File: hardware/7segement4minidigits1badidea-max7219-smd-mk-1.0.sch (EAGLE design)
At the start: 12 parts, among them IC1 MAX7219

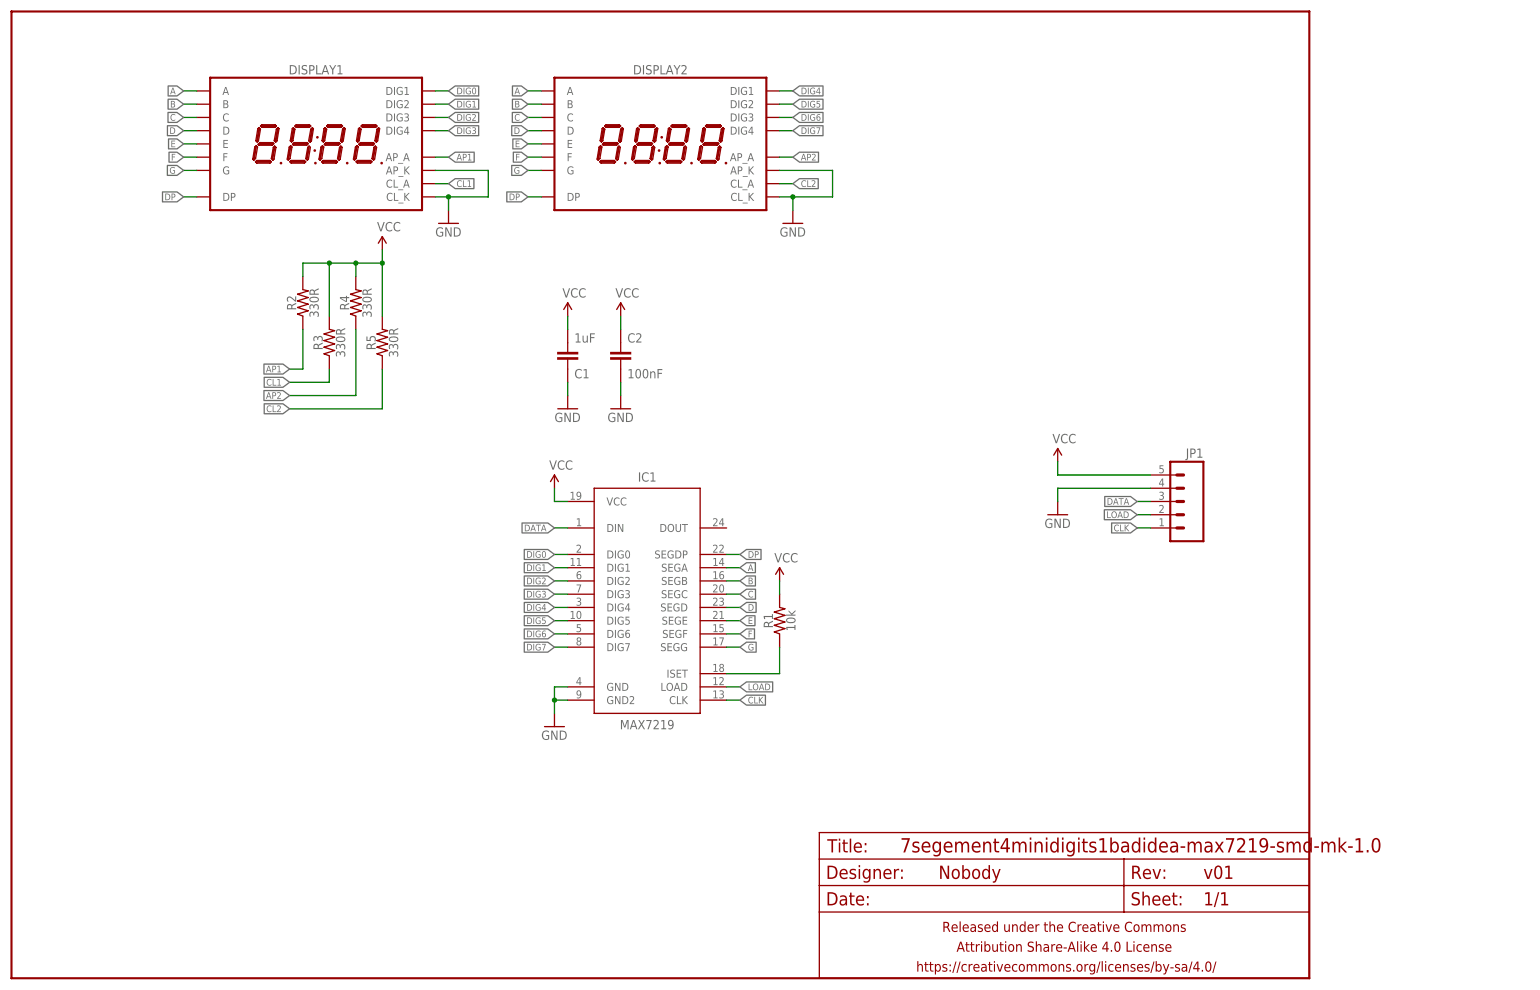
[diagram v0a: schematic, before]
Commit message: whooooole bunch of designs i apparently never committed
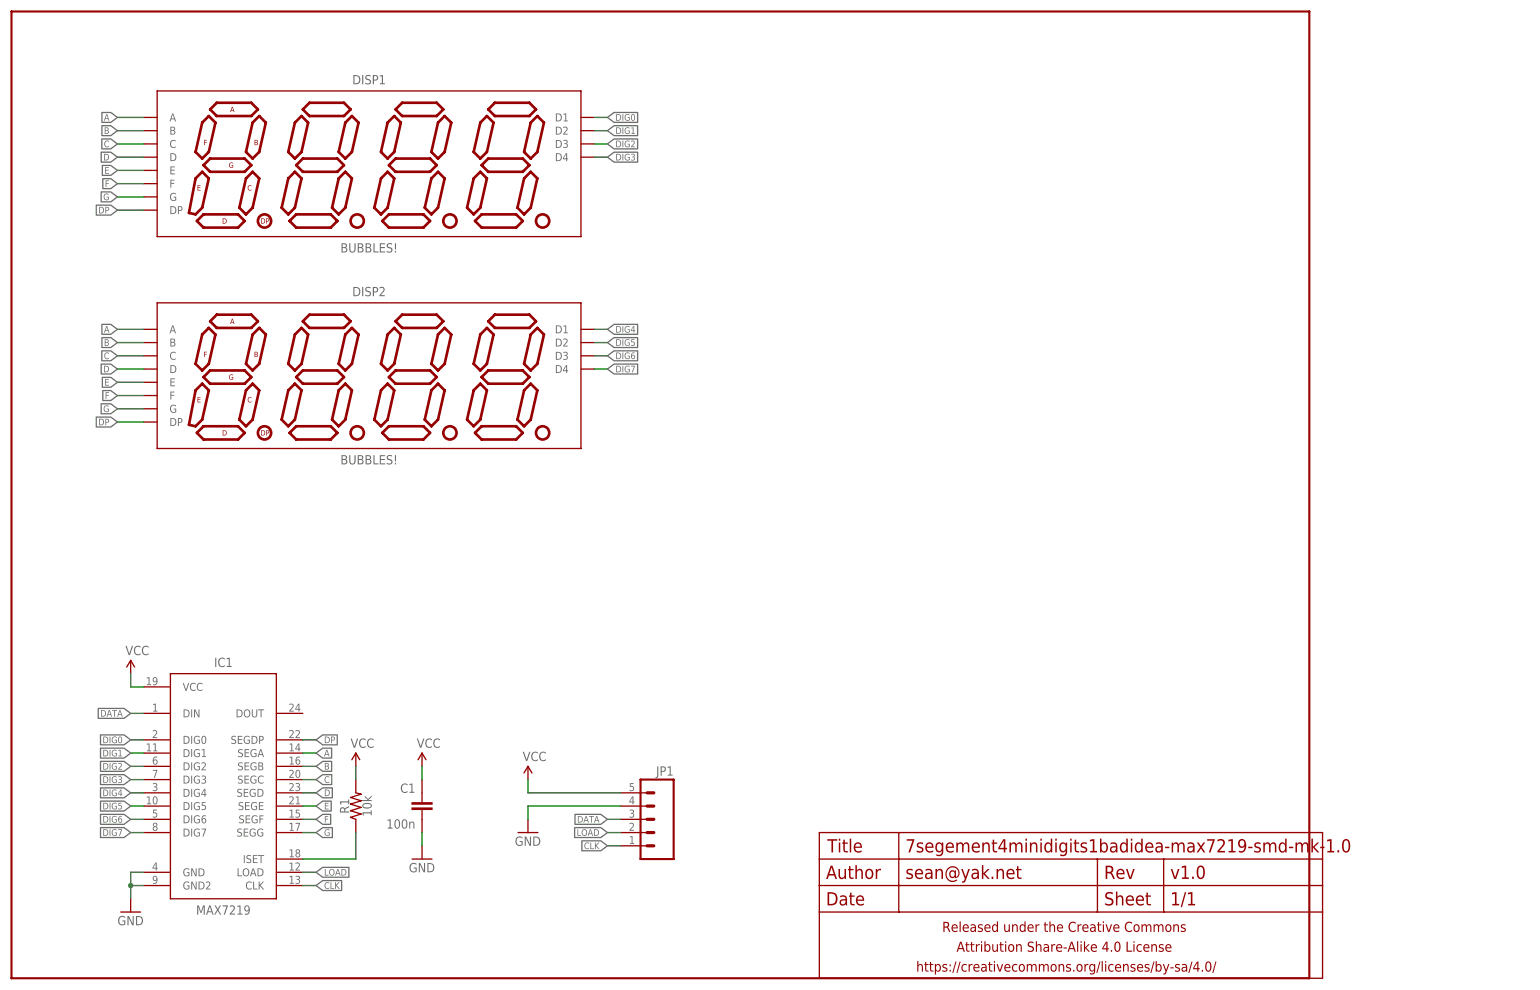
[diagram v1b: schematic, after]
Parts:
- removed C2: 100nF, A_butts:CAPACITOR-CERAMICC0805
- removed DISPLAY1, DISPLAY2: 7SEG_4DIGIT_COLON_APOS, A_butts:7SEG_4DIGIT_COLON_APOS
- removed R2, R3, R4, R5: 330R, A_butts:RESISTORR0805
- added DISP1, DISP2: BUBBLES!, A_butts:7SEG_4DIGITHP-BUBBLE
- C1: value 1uF -> 100n; device A_butts:CAPACITOR-CERAMICC0805 -> A_butts:CAPACITOR-CERAMICC0603
- FRAME1: DESIGNER (none) -> sean@yak.net; VERSION (none) -> v1.0
- JP1: value M05PTH -> M05PTH-CENTERED; device A_butts:M05PTH -> A_butts:M05PTH-CENTERED
- R1: device A_butts:RESISTORR0805 -> A_butts:RESISTORR0603
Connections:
- removed net AP1: DISPLAY1.AP_A, R2.1
- removed net AP2: DISPLAY2.AP_A, R4.1
- removed net CL1: DISPLAY1.CL_A, R3.1
- removed net CL2: DISPLAY2.CL_A, R5.1
- net A: now also DISP1.A, DISP2.A; no longer DISPLAY1.A, DISPLAY2.A
- net B: now also DISP1.B, DISP2.B; no longer DISPLAY1.B, DISPLAY2.B
- net C: now also DISP1.C, DISP2.C; no longer DISPLAY1.C, DISPLAY2.C
- net D: now also DISP1.D, DISP2.D; no longer DISPLAY1.D, DISPLAY2.D
- net DIG0: now also DISP1.D1; no longer DISPLAY1.DIG1
- net DIG1: now also DISP1.D2; no longer DISPLAY1.DIG2
- net DIG2: now also DISP1.D3; no longer DISPLAY1.DIG3
- net DIG3: now also DISP1.D4; no longer DISPLAY1.DIG4
- net DIG4: now also DISP2.D1; no longer DISPLAY2.DIG1
- net DIG5: now also DISP2.D2; no longer DISPLAY2.DIG2
- net DIG6: now also DISP2.D3; no longer DISPLAY2.DIG3
- net DIG7: now also DISP2.D4; no longer DISPLAY2.DIG4
- net DP: now also DISP1.DP, DISP2.DP; no longer DISPLAY1.DP, DISPLAY2.DP
- net E: now also DISP1.E, DISP2.E; no longer DISPLAY1.E, DISPLAY2.E
- net F: now also DISP1.F, DISP2.F; no longer DISPLAY1.F, DISPLAY2.F
- net G: now also DISP1.G, DISP2.G; no longer DISPLAY1.G, DISPLAY2.G
- net GND: now also C1.2; no longer C1.1, C2.2, DISPLAY1.AP_K, DISPLAY1.CL_K, DISPLAY2.AP_K, DISPLAY2.CL_K
- net VCC: now also C1.1; no longer C1.2, C2.1, R2.2, R3.2, R4.2, R5.2
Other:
- moved on the sheet: C1, IC1, JP1, R1
